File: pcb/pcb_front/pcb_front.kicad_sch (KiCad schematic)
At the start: 8 parts, among them J1 MicroLab, J2 Sensors, J3 LED

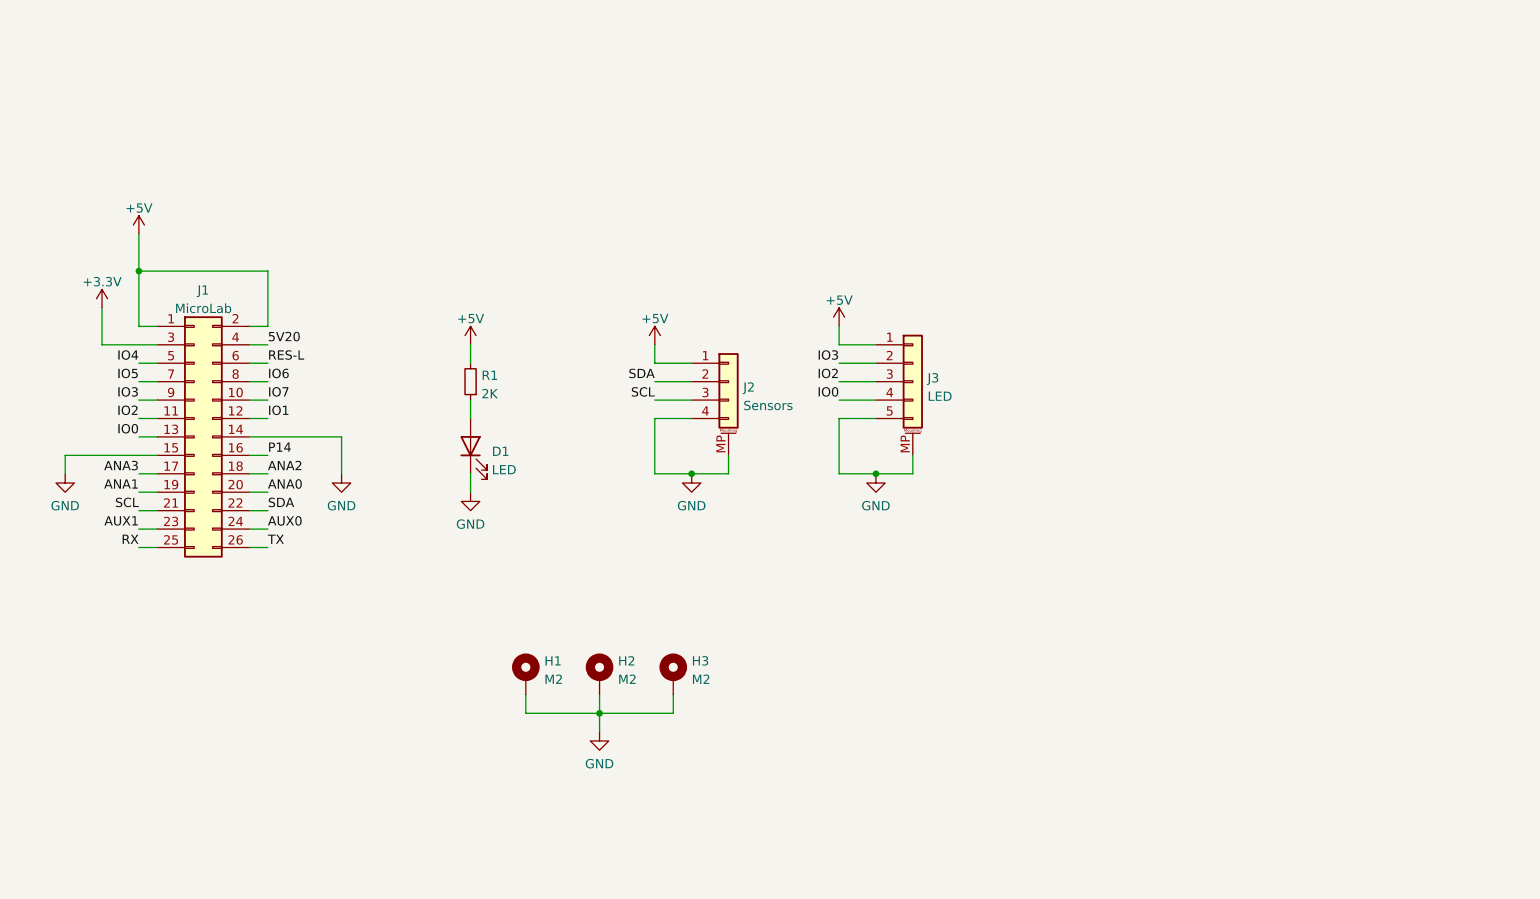
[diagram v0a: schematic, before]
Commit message: production ver. of PCB
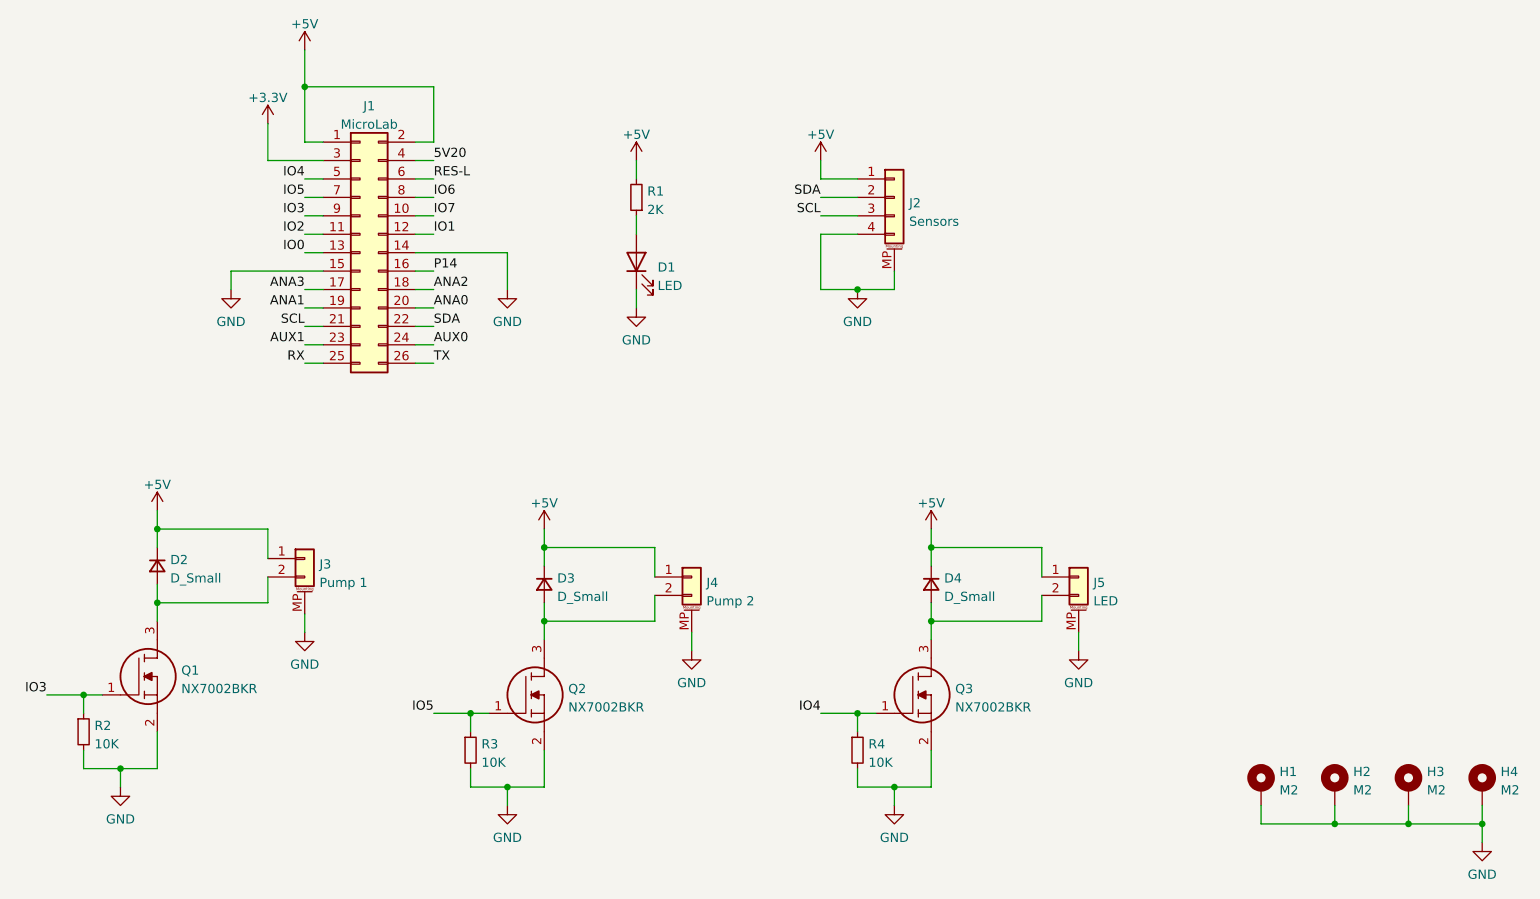
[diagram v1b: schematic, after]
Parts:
- removed J3: LED, Connector_JST:JST_SH_BM05B-SRSS-TB_1x05-1MP_P1.00mm_Vertical, symbol Connector_Generic_MountingPin:Conn_01x05_MountingPin
- added D2, D3, D4: D_Small, Diode_SMD:D_SOD-323, symbol Device:D_Small
- added H4: M2, MountingHole:MountingHole_2.2mm_M2_DIN965_Pad, symbol Mechanical:MountingHole_Pad
- added J3: Pump 1, Connector_JST:JST_SH_BM02B-SRSS-TB_1x02-1MP_P1.00mm_Vertical, symbol Connector_Generic_MountingPin:Conn_01x02_MountingPin
- added J4: Pump 2, Connector_JST:JST_SH_BM02B-SRSS-TB_1x02-1MP_P1.00mm_Vertical, symbol Connector_Generic_MountingPin:Conn_01x02_MountingPin
- added J5: LED, Connector_JST:JST_SH_BM02B-SRSS-TB_1x02-1MP_P1.00mm_Vertical, symbol Connector_Generic_MountingPin:Conn_01x02_MountingPin
- added Q1, Q2, Q3: NX7002BKR, SOT95P230X110-3N, symbol Mouser Parts:NX7002BKR
- added R2, R3, R4: 10K, Resistor_SMD:R_0402_1005Metric, symbol Device:R_Small
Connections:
- net +5V: now also D2.1 (K), D3.1 (K), D4.1 (K), J3.1 (Pin_1), J4.1 (Pin_1), J5.1 (Pin_1)
- net GND: now also H4.1, J3.MP (MountPin), J4.MP (MountPin), J5.MP (MountPin), Q1.2, Q2.2, Q3.2, R2.2, R3.2, R4.2
- net IO3: now also Q1.1, R2.1
- net IO4: now also Q3.1, R4.1
- net IO5: now also Q2.1, R3.1
- new net: D4.2 (A), J5.2 (Pin_2), Q3.3
- new net: D3.2 (A), J4.2 (Pin_2), Q2.3
- new net: D2.2 (A), J3.2 (Pin_2), Q1.3
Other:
- moved on the sheet: D1, H1, H2, H3, J1, J2, R1
